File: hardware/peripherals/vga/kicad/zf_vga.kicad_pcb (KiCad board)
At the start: 2 copper layers, 33 parts, among them J2 Conn_02x13_Odd_Even, J3 DB15_Female, J4 DB9_Male, J5 DB9_Male, SW1 SW_DIP_x03, U1 4040, U10 74HC165, U11 AS6C6264, U12 74HC541, U13 74HC541, U14 74HC541, U2 4040, U3 GAL16V8, U4 GAL16V8, U5 74HC541, U6 74HC541, U7 74HC00, U8 74HC04, U9 74HC74, X1 CXO_DIP14

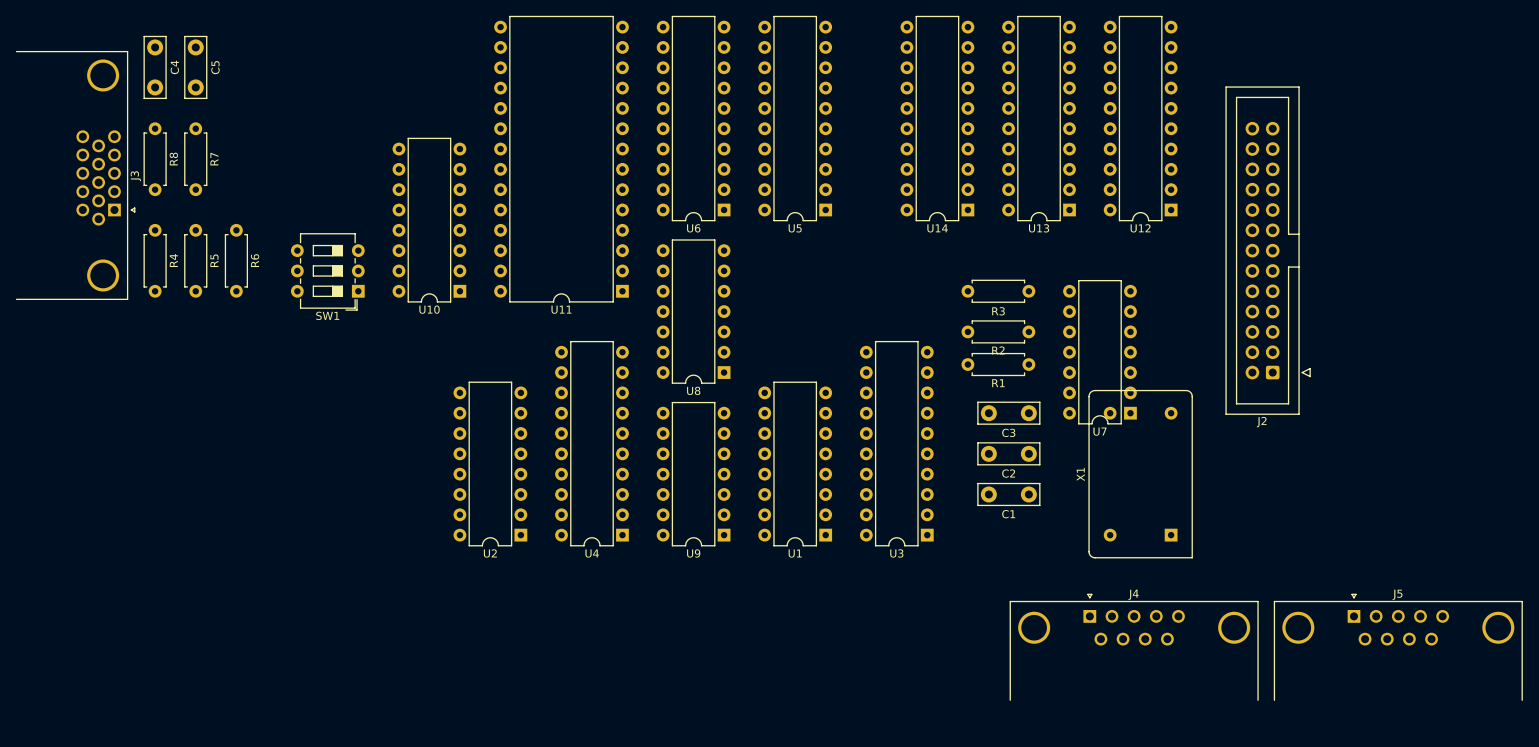
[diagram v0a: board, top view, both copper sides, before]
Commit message: Bypass caps
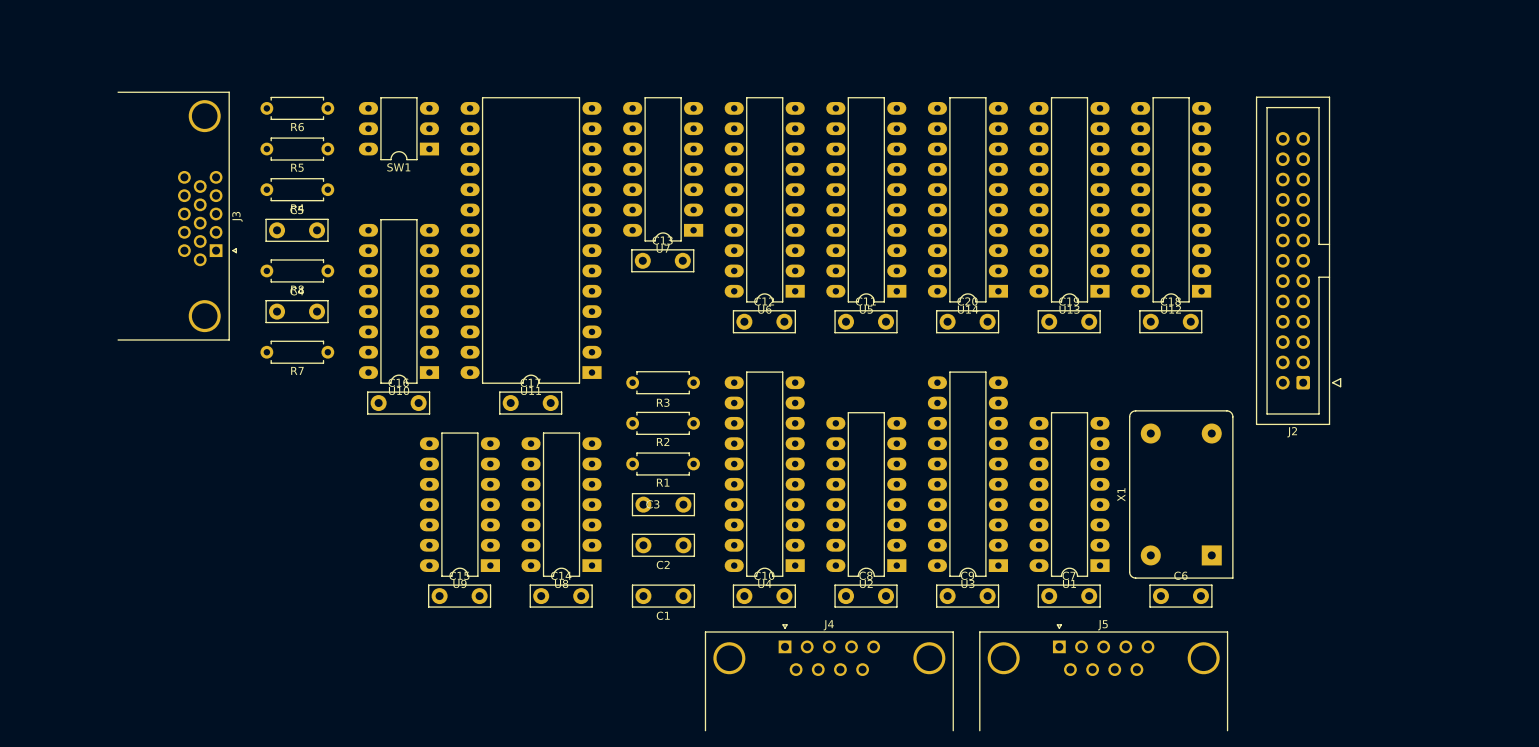
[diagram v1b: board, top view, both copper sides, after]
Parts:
- added C10: 0.1uF, Capacitor_THT:C_Disc_D7.5mm_W2.5mm_P5.00mm, F.Cu at (149.9, 116.8)
- added C11: 0.1uF, Capacitor_THT:C_Disc_D7.5mm_W2.5mm_P5.00mm, F.Cu at (162.6, 82.5)
- added C12: 0.1uF, Capacitor_THT:C_Disc_D7.5mm_W2.5mm_P5.00mm, F.Cu at (149.9, 82.5)
- added C13: 0.1uF, Capacitor_THT:C_Disc_D7.5mm_W2.5mm_P5.00mm, F.Cu at (137.2, 74.9)
- added C14: 0.1uF, Capacitor_THT:C_Disc_D7.5mm_W2.5mm_P5.00mm, F.Cu at (124.5, 116.8)
- added C15: 0.1uF, Capacitor_THT:C_Disc_D7.5mm_W2.5mm_P5.00mm, F.Cu at (111.8, 116.8)
- added C16: 0.1uF, Capacitor_THT:C_Disc_D7.5mm_W2.5mm_P5.00mm, F.Cu at (104.1, 92.7)
- added C17: 0.1uF, Capacitor_THT:C_Disc_D7.5mm_W2.5mm_P5.00mm, F.Cu at (120.7, 92.7)
- added C18: 0.1uF, Capacitor_THT:C_Disc_D7.5mm_W2.5mm_P5.00mm, F.Cu at (200.7, 82.5)
- added C19: 0.1uF, Capacitor_THT:C_Disc_D7.5mm_W2.5mm_P5.00mm, F.Cu at (188.0, 82.5)
- added C20: 0.1uF, Capacitor_THT:C_Disc_D7.5mm_W2.5mm_P5.00mm, F.Cu at (175.3, 82.5)
- added C6: 0.1uF, Capacitor_THT:C_Disc_D7.5mm_W2.5mm_P5.00mm, F.Cu at (201.9, 116.8)
- added C7: 0.1uF, Capacitor_THT:C_Disc_D7.5mm_W2.5mm_P5.00mm, F.Cu at (188.0, 116.8)
- added C8: 0.1uF, Capacitor_THT:C_Disc_D7.5mm_W2.5mm_P5.00mm, F.Cu at (162.6, 116.8)
- added C9: 0.1uF, Capacitor_THT:C_Disc_D7.5mm_W2.5mm_P5.00mm, F.Cu at (175.3, 116.8)
- SW1: footprint Button_Switch_THT:SW_DIP_SPSTx03_Slide_6.7x9.18mm_W7.62mm_P2.54mm_LowProfile -> Package_DIP:DIP-6_W7.62mm_LongPads
- U1, U10, U2: footprint Package_DIP:DIP-16_W7.62mm -> Package_DIP:DIP-16_W7.62mm_LongPads
- U11: footprint Package_DIP:DIP-28_W15.24mm -> Package_DIP:DIP-28_W15.24mm_LongPads
- U12, U13, U14, U3, U4, U5, U6: footprint Package_DIP:DIP-20_W7.62mm -> Package_DIP:DIP-20_W7.62mm_LongPads
- U7, U8, U9: footprint Package_DIP:DIP-14_W7.62mm -> Package_DIP:DIP-14_W7.62mm_LongPads
- X1: footprint Oscillator:Oscillator_DIP-14 -> Oscillator:Oscillator_DIP-14_LargePads
- moved U7 59.2 mm to (143.5, 71.1)
- moved U2 47.1 mm to (168.9, 113.0)
- moved C1 45.0 mm to (142.2, 116.8)
- moved C2 44.7 mm to (142.2, 110.5)
- moved C3 44.7 mm to (142.2, 105.4)
- moved R1 43.7 mm to (143.5, 100.3)
- moved R2 43.4 mm to (143.5, 95.2)
- moved R3 43.4 mm to (143.5, 90.2)
- moved J4 38.3 mm to (154.9, 123.2)
- moved J5 37.0 mm to (189.2, 123.2)
- moved C4 36.4 mm to (91.4, 81.3), turned to 0 degrees
- moved U1 34.5 mm to (194.3, 113.0)
- moved R7 32.5 mm to (97.8, 86.4), turned to 180 degrees
- moved U9 29.5 mm to (118.1, 113.0)
- moved U8 29.2 mm to (130.8, 113.0)
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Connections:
- C4 pad 1: GND -> Net-(C4-Pad1)
- C4 pad 2: Net-(C4-Pad2) -> GND
- C5 pad 1: GND -> Net-(C5-Pad1)
- C5 pad 2: Net-(C4-Pad2) -> GND
- J3 pad 13: Net-(J3-Pad13) -> Net-(C4-Pad1)
- J3 pad 14: Net-(C4-Pad2) -> Net-(C5-Pad1)
- R7 pad 2: Net-(J3-Pad13) -> Net-(C4-Pad1)
- R8 pad 2: Net-(C4-Pad2) -> Net-(C5-Pad1)
- U12 pad 11: D7 -> D0
- U12 pad 12: D6 -> D1
- U12 pad 13: D5 -> D2
- U12 pad 14: D4 -> D3
- U12 pad 15: D3 -> D4
- U12 pad 16: D2 -> D5
- U12 pad 17: D1 -> D6
- U12 pad 18: D0 -> D7
- U12 pad 2: PA0 -> PA7
- U12 pad 3: PA1 -> PA6
- U12 pad 4: PA2 -> PA5
- U12 pad 5: PA3 -> PA4
- U12 pad 6: PA4 -> PA3
- U12 pad 7: PA5 -> PA2
- U12 pad 8: PA6 -> PA1
- U12 pad 9: PA7 -> PA0
- U13 pad 11: A7 -> A0
- U13 pad 12: A6 -> A1
- U13 pad 13: A5 -> A2
- U13 pad 14: A4 -> A3
- U13 pad 15: A3 -> A4
- U13 pad 16: A2 -> A5
- U13 pad 17: A1 -> A6
- U13 pad 18: A0 -> A7
- U13 pad 2: PB0 -> PB7
- U13 pad 3: PB1 -> PB6
- U13 pad 4: PB2 -> PB5
- U13 pad 5: PB3 -> PB4
- U13 pad 6: PB4 -> PB3
- U13 pad 7: PB5 -> PB2
- U13 pad 8: PB6 -> PB1
- U13 pad 9: PB7 -> PB0
- U14 pad 16: A10 -> A8
- U14 pad 18: A8 -> A10
- U14 pad 2: PC0 -> PC2
- U14 pad 4: PC2 -> PC0
- U3 pad 1: P0 -> P9
- U3 pad 11: P9 -> P0
- U3 pad 2: P1 -> P8
- U3 pad 3: P2 -> P7
- U3 pad 4: P3 -> P6
- U3 pad 5: P4 -> P5
- U3 pad 6: P5 -> P4
- U3 pad 7: P6 -> P3
- U3 pad 8: P7 -> P2
- U3 pad 9: P8 -> P1
- U4 pad 1: L0 -> L9
- U4 pad 11: L9 -> L0
- U4 pad 2: L1 -> L8
- U4 pad 3: L2 -> L7
- U4 pad 4: L3 -> L6
- U4 pad 5: L4 -> L5
- U4 pad 6: L5 -> L4
- U4 pad 7: L6 -> L3
- U4 pad 8: L7 -> L2
- U4 pad 9: L8 -> L1
- U5 pad 15: A3 -> A0
- U5 pad 16: A2 -> A1
- U5 pad 17: A1 -> A2
- U5 pad 18: A0 -> A3
- U5 pad 2: P5 -> P8
- U5 pad 3: P6 -> P7
- U5 pad 4: P7 -> P6
- U5 pad 5: P8 -> P5
- U6 pad 12: A10 -> A4
- U6 pad 13: A9 -> A5
- U6 pad 14: A8 -> A6
- U6 pad 16: A6 -> A8
- U6 pad 17: A5 -> A9
- U6 pad 18: A4 -> A10
- U6 pad 2: L2 -> L8
- U6 pad 3: L3 -> L7
- U6 pad 4: L4 -> L6
- U6 pad 6: L6 -> L4
- U6 pad 7: L7 -> L3
- U6 pad 8: L8 -> L2
